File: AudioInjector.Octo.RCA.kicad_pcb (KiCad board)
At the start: 2 copper layers, 58.5 x 43.9 mm, 66 parts, among them P5 DAC_out, P6 ADC_in, U20 AV6-8.4-13, U21 AV8-8.4-13

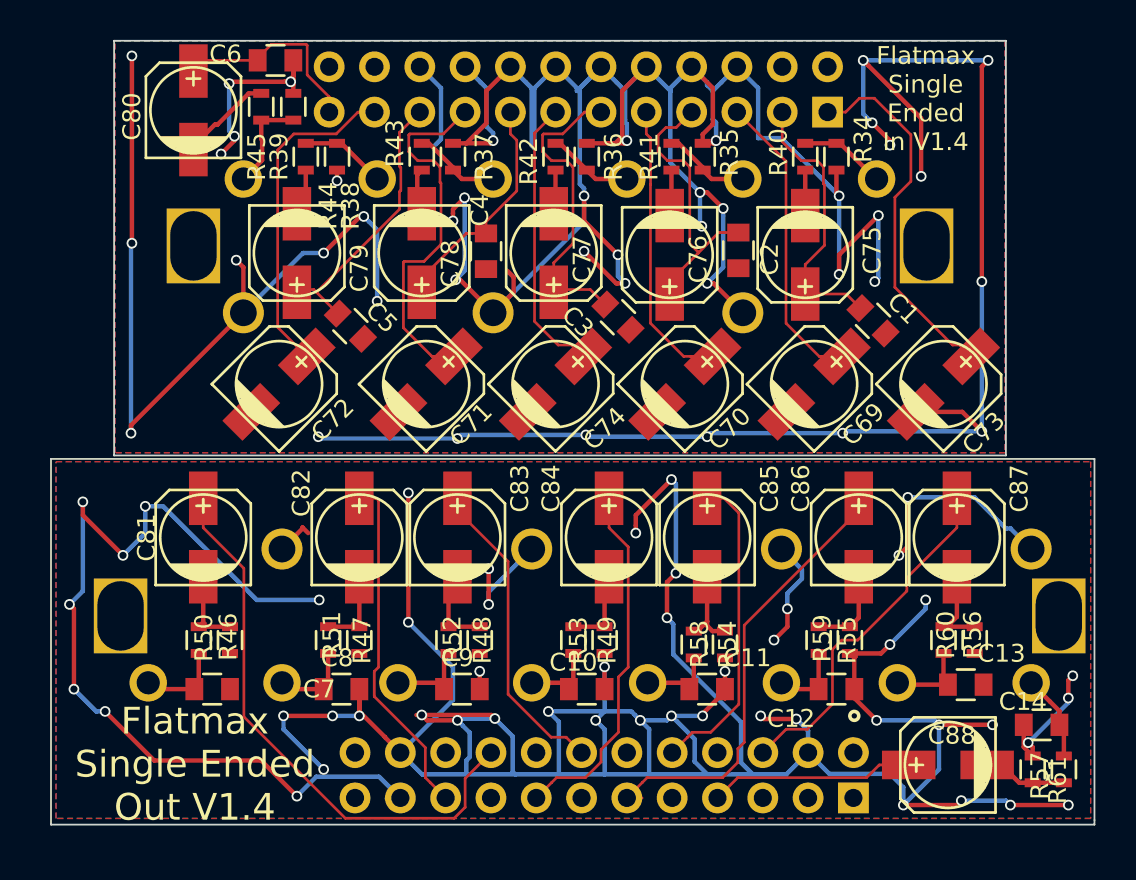
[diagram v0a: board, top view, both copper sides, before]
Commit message: Adding v1.5 of these PCBs.
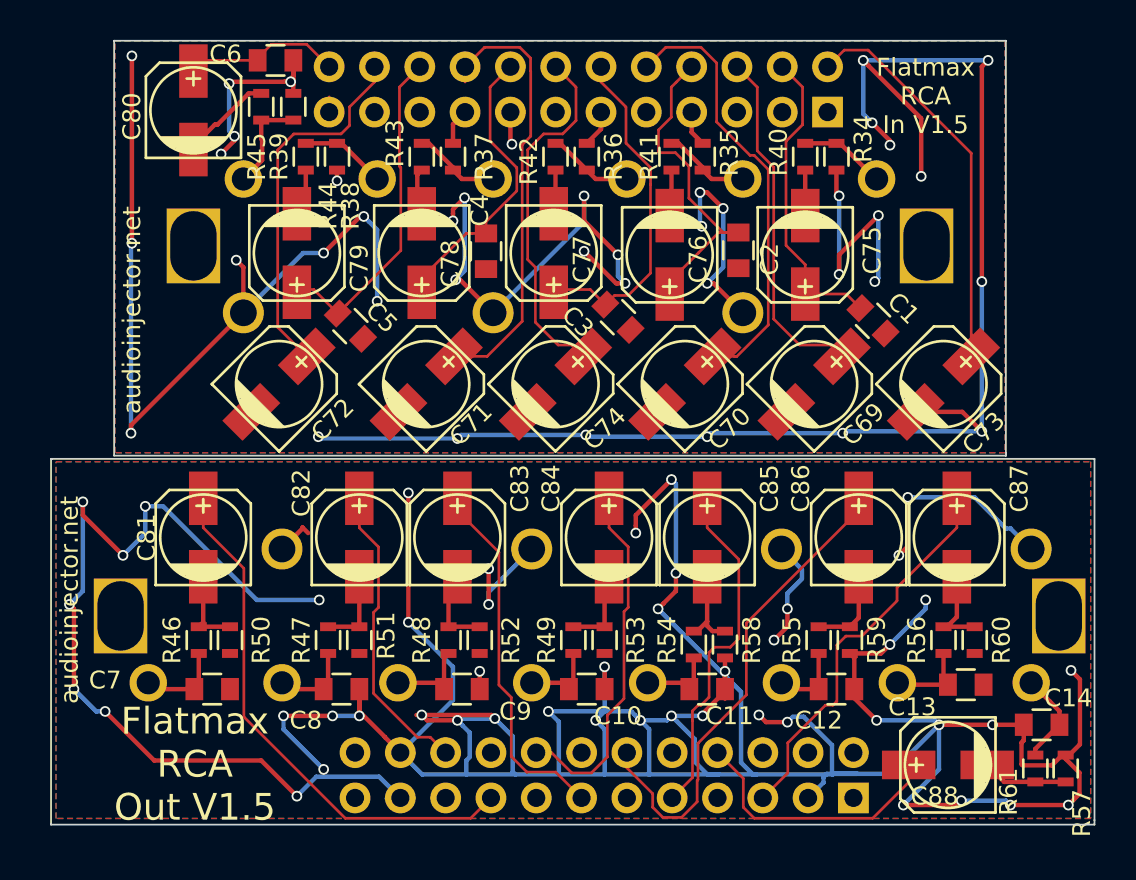
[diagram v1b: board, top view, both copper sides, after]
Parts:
- moved R61 1.85 mm to (173.8, 167.4)
- moved R57 1.60 mm to (172.2, 167.4)
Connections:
- P5 pad 10: /Codec/AOUT5+ -> (no net)
- P5 pad 11: /Codec/AOUT6+ -> (no net)
- P5 pad 12: (no net) -> /Codec/AOUT6+
- P5 pad 13: (no net) -> /Codec/AOUT3+
- P5 pad 14: /Codec/AOUT3+ -> (no net)
- P5 pad 15: /Codec/AOUT4+ -> (no net)
- P5 pad 16: (no net) -> /Codec/AOUT4+
- P5 pad 17: (no net) -> /Codec/AOUT1+
- P5 pad 18: /Codec/AOUT1+ -> (no net)
- P5 pad 19: /Codec/AOUT2+ -> (no net)
- P5 pad 20: (no net) -> /Codec/AOUT2+
- P5 pad 3: (no net) -> /Codec/AGND
- P5 pad 4: /Codec/AGND -> (no net)
- P5 pad 5: (no net) -> /Codec/AOUT7+
- P5 pad 6: /Codec/AOUT7+ -> (no net)
- P5 pad 7: /Codec/AOUT8+ -> (no net)
- P5 pad 8: (no net) -> /Codec/AOUT8+
- P5 pad 9: (no net) -> /Codec/AOUT5+
- P6 pad 1: /Codec/ADC_fb1- -> V5
- P6 pad 10: /Codec/AGND -> /Codec/ADC_fb3-
- P6 pad 11: /Codec/ADC_fb3+ -> /Codec/AGND
- P6 pad 12: /Codec/AGND -> /Codec/ADC_fb3+
- P6 pad 13: /Codec/ADC_fb4- -> /Codec/AGND
- P6 pad 14: /Codec/AGND -> /Codec/ADC_fb4-
- P6 pad 15: /Codec/ADC_fb4+ -> /Codec/AGND
- P6 pad 16: /Codec/AGND -> /Codec/ADC_fb4+
- P6 pad 17: /Codec/ADC_fb5- -> /Codec/AGND
- P6 pad 18: /Codec/AGND -> /Codec/ADC_fb5-
- P6 pad 19: /Codec/ADC_fb5+ -> /Codec/AGND
- P6 pad 2: V5 -> /Codec/ADC_fb1-
- P6 pad 20: /Codec/AGND -> /Codec/ADC_fb5+
- P6 pad 21: /Codec/ADC_fb6- -> V5
- P6 pad 22: V5 -> /Codec/ADC_fb6-
- P6 pad 23: /Codec/ADC_fb6+ -> V5
- P6 pad 24: V5 -> /Codec/ADC_fb6+
- P6 pad 3: /Codec/ADC_fb1+ -> V5
- P6 pad 4: V5 -> /Codec/ADC_fb1+
- P6 pad 5: /Codec/ADC_fb2- -> /Codec/AGND
- P6 pad 6: /Codec/AGND -> /Codec/ADC_fb2-
- P6 pad 7: /Codec/ADC_fb2+ -> /Codec/AGND
- P6 pad 8: /Codec/AGND -> /Codec/ADC_fb2+
- P6 pad 9: /Codec/ADC_fb3- -> /Codec/AGND
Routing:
- net /Codec/AGND: track 542.5 -> 476.1 mm, vias 91 -> 87
- net /Codec/ADC_fb3-: track 16.2 -> 24.6 mm
- net /Codec/ADC_fb4-: track 15.8 -> 20.2 mm
- net /Codec/ADC_fb5-: track 20.8 -> 24.8 mm
- net /Codec/AOUT8+: track 11.5 -> 15.0 mm
- net /Codec/ADC_fb4+: track 14.0 -> 17.4 mm
- net /Codec/ADC_fb5+: track 16.1 -> 19.4 mm
- net /Codec/AOUT3+: track 17.6 -> 20.6 mm
- net /Codec/ADC_fb2-: track 16.9 -> 19.7 mm
- net /Codec/AOUT2+: track 20.3 -> 17.6 mm
- net /Codec/ADC_fb6+: track 11.4 -> 8.83 mm
- net /Codec/ADC_fb2+: track 16.2 -> 18.6 mm
- net /Codec/ADC_fb6-: track 18.5 -> 20.7 mm
- net /Codec/AOUT7+: track 20.7 -> 22.8 mm
- net /Codec/AOUT6+: track 25.5 -> 27.5 mm
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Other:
- outline, holes or cut-outs redrawn
- board text added: "Flatmax RCA In V1.5"
- board text added: "Flatmax RCA Out V1.5"
- board text added: "audioinjector.net"
- board text removed: "Flatmax Single Ended In V1.4"
- board text removed: "Flatmax Single Ended Out V1.4"
